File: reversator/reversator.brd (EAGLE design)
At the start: 6 parts

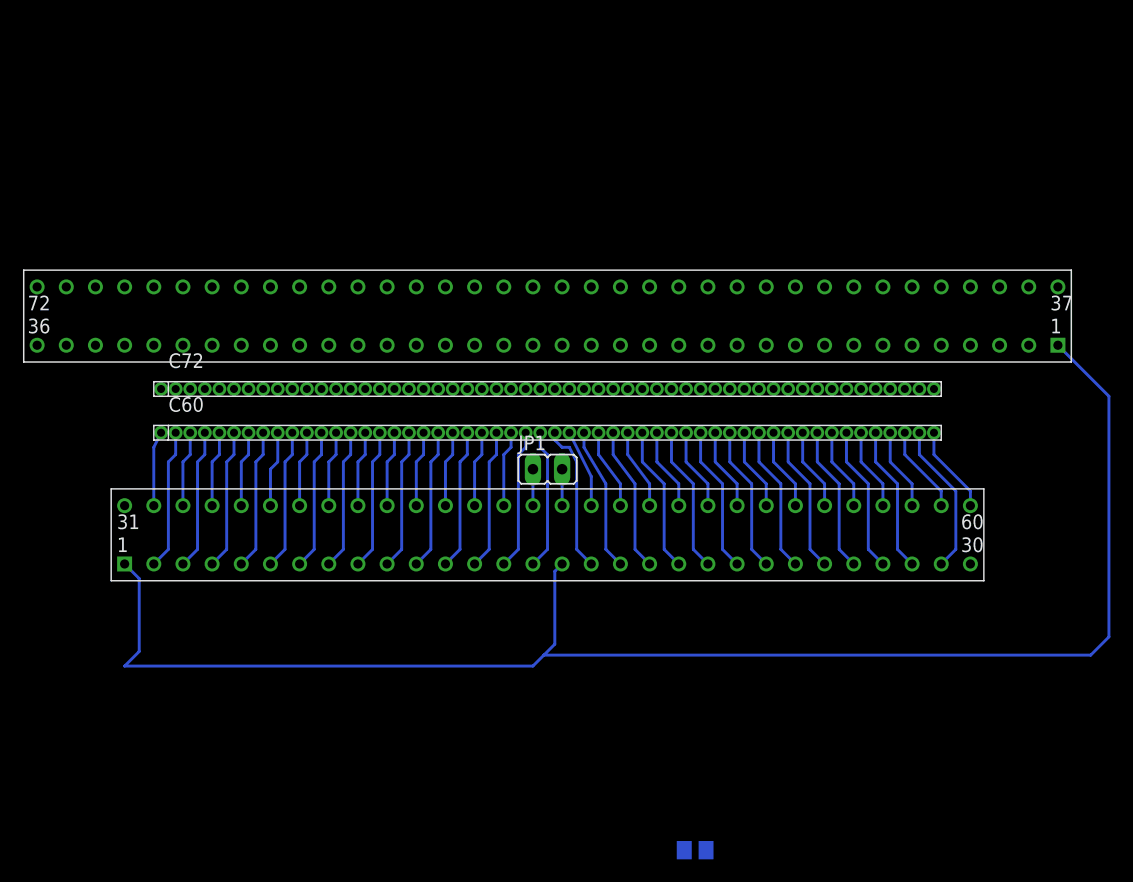
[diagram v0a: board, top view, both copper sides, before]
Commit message: .
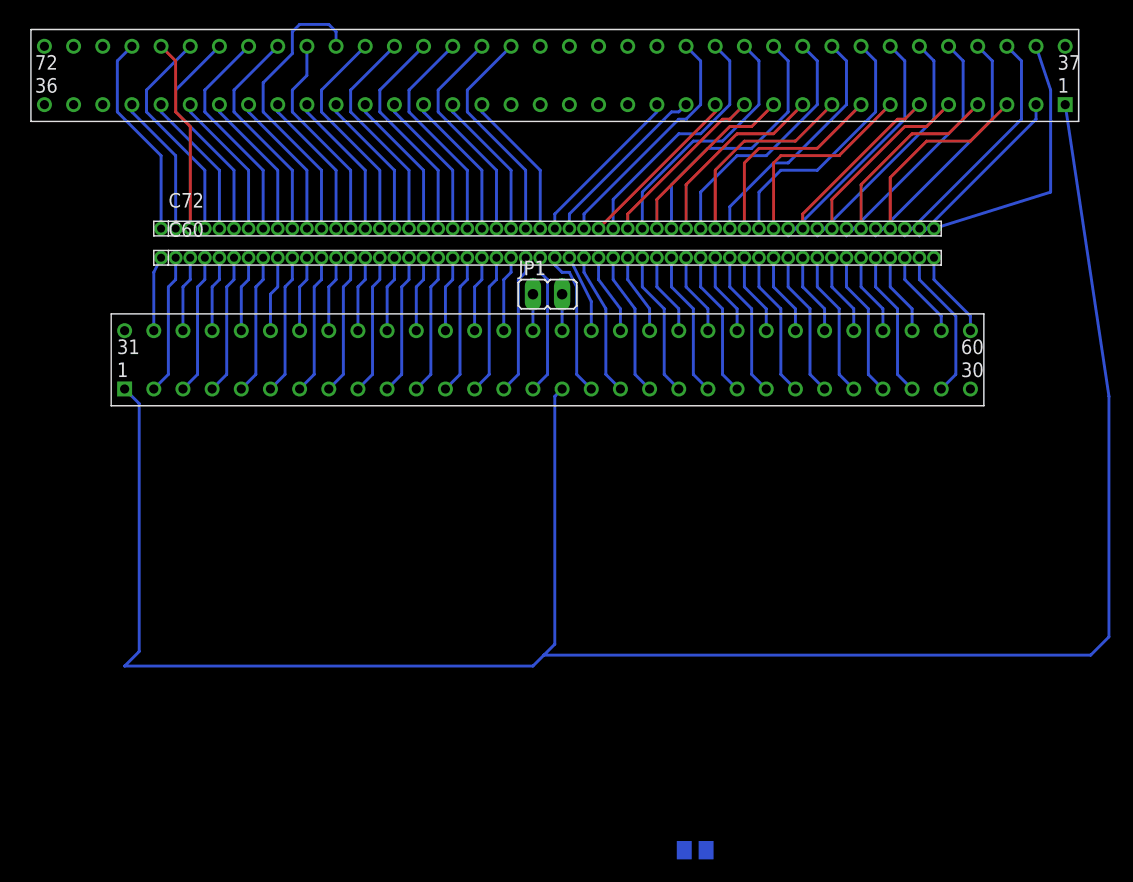
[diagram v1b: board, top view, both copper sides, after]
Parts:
- moved SLOT_N 21.0 mm to (0.64, 40.0)
- moved SLOT_F 15.2 mm to (0.00, 15.2)
- moved C60 15.2 mm to (0.00, 24.1)
- moved JP1 15.2 mm to (0.00, 21.0)
- moved C72 14.0 mm to (0.00, 26.7)
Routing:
- net GND: track 132.6 -> 182.4 mm
- net PA11: track 7.14 -> 33.0 mm
- net M2: track 6.50 -> 30.1 mm
- net D2: track 6.61 -> 29.5 mm
- net D5: track 6.61 -> 29.1 mm
- net D3: track 6.61 -> 28.7 mm
- net D1: track 6.61 -> 28.7 mm
- net D7: track 6.61 -> 28.5 mm
- net D6: track 6.61 -> 28.5 mm
- net A14: track 6.61 -> 28.5 mm
- net A13: track 6.61 -> 28.5 mm
- net A12: track 6.61 -> 28.5 mm
- net D0: track 6.61 -> 28.3 mm
- net D4: track 6.61 -> 28.0 mm
- net !ROMSEL: track 6.61 -> 27.6 mm
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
